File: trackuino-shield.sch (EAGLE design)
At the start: 19 parts, among them IC2 AP1117, M1 HX1, Q1 IRLD110, U1 LM60 int, X1 BU-SMA-V, X2 Vin, X3 LM60 ext, X4 Buzzer

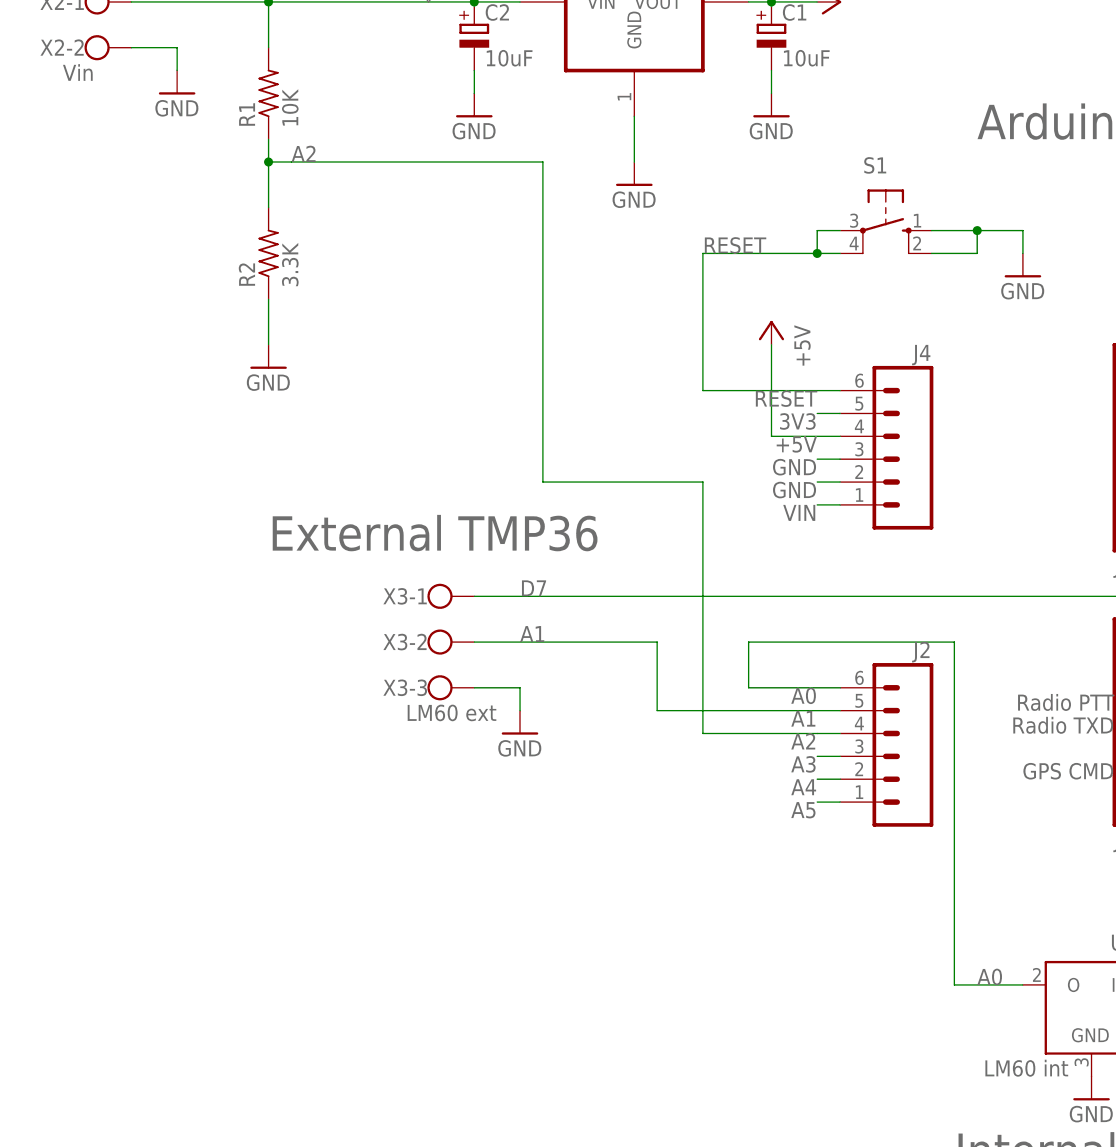
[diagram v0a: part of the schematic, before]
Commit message: Added logo
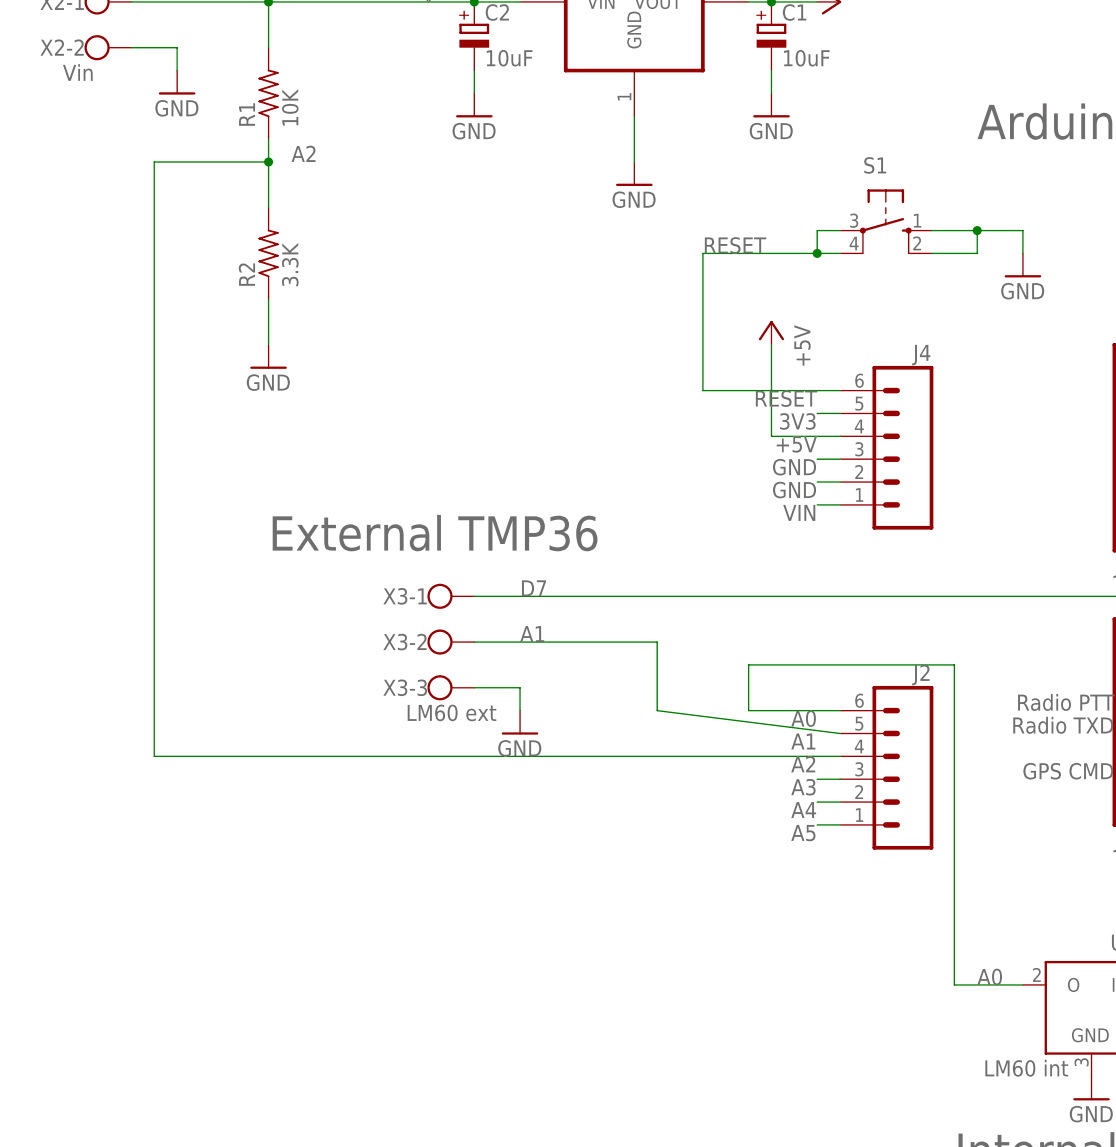
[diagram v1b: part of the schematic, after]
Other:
- moved on the sheet: J2
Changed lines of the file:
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@@
 <instance part="S1" gate="1" x="99.06" y="137.16" rot="R270"/>
 <instance part="J4" gate="G$1" x="99.06" y="111.76" rot="MR0"/>
-<instance part="J2" gate="G$1" x="99.06" y="78.74" rot="MR0"/>
+<instance part="J2" gate="G$1" x="99.06" y="76.2" rot="MR0"/>
 <instance part="J3" gate="G$1" x="129.54" y="114.3" rot="MR180"/>
 <instance part="J1" gate="G$1" x="129.54" y="83.82" rot="MR180"/>
@@
 <pinref part="U1" gate="G$1" pin="O"/>
 <wire x1="114.3" y1="53.34" x2="106.68" y2="53.34" width="0.1524" layer="91"/>
-<wire x1="93.98" y1="86.36" x2="83.82" y2="86.36" width="0.1524" layer="91"/>
-<label x="91.44" y="86.36" size="1.778" layer="95" rot="R180"/>
+<wire x1="93.98" y1="83.82" x2="83.82" y2="83.82" width="0.1524" layer="91"/>
+<label x="91.44" y="83.82" size="1.778" layer="95" rot="R180"/>
 <pinref part="J2" gate="G$1" pin="6"/>
-<wire x1="106.68" y1="53.34" x2="106.68" y2="91.44" width="0.1524" layer="91"/>
-<wire x1="106.68" y1="91.44" x2="83.82" y2="91.44" width="0.1524" layer="91"/>
-<wire x1="83.82" y1="91.44" x2="83.82" y2="86.36" width="0.1524" layer="91"/>
+<wire x1="106.68" y1="53.34" x2="106.68" y2="88.9" width="0.1524" layer="91"/>
+<wire x1="106.68" y1="88.9" x2="83.82" y2="88.9" width="0.1524" layer="91"/>
+<wire x1="83.82" y1="88.9" x2="83.82" y2="83.82" width="0.1524" layer="91"/>
 </segment>
 </net>
@@
 <wire x1="53.34" y1="91.44" x2="73.66" y2="91.44" width="0.1524" layer="91"/>
 <wire x1="73.66" y1="91.44" x2="73.66" y2="83.82" width="0.1524" layer="91"/>
-<label x="91.44" y="83.82" size="1.778" layer="95" rot="R180"/>
+<label x="91.44" y="81.28" size="1.778" layer="95" rot="R180"/>
 <pinref part="J2" gate="G$1" pin="5"/>
-<wire x1="73.66" y1="83.82" x2="93.98" y2="83.82" width="0.1524" layer="91"/>
+<wire x1="73.66" y1="83.82" x2="93.98" y2="81.28" width="0.1524" layer="91"/>
 </segment>
 </net>
@@
 <wire x1="30.48" y1="147.32" x2="30.48" y2="144.78" width="0.1524" layer="91"/>
 <wire x1="30.48" y1="144.78" x2="30.48" y2="139.7" width="0.1524" layer="91"/>
-<wire x1="30.48" y1="144.78" x2="33.02" y2="144.78" width="0.1524" layer="91"/>
 <junction x="30.48" y="144.78"/>
 <label x="33.02" y="144.78" size="1.778" layer="95"/>
 <pinref part="R1" gate="G$1" pin="1"/>
 <pinref part="R2" gate="G$1" pin="2"/>
-<wire x1="33.02" y1="144.78" x2="60.96" y2="144.78" width="0.2032" layer="91"/>
-<wire x1="60.96" y1="144.78" x2="60.96" y2="109.22" width="0.2032" layer="91"/>
-<wire x1="60.96" y1="109.22" x2="78.74" y2="109.22" width="0.2032" layer="91"/>
-<wire x1="78.74" y1="109.22" x2="78.74" y2="81.28" width="0.2032" layer="91"/>
-<wire x1="78.74" y1="81.28" x2="91.44" y2="81.28" width="0.2032" layer="91"/>
-<wire x1="93.98" y1="81.28" x2="91.44" y2="81.28" width="0.1524" layer="91"/>
-<label x="91.44" y="81.28" size="1.778" layer="95" rot="R180"/>
+<wire x1="30.48" y1="144.78" x2="17.78" y2="144.78" width="0.1524" layer="91"/>
+<wire x1="17.78" y1="144.78" x2="17.78" y2="78.74" width="0.1524" layer="91"/>
+<wire x1="17.78" y1="78.74" x2="93.98" y2="78.74" width="0.1524" layer="91"/>
+<label x="91.44" y="78.74" size="1.778" layer="95" rot="R180"/>
 <pinref part="J2" gate="G$1" pin="4"/>
 </segment>
 </net>
 <net name="A3" class="0">
-<segment>
-<wire x1="93.98" y1="78.74" x2="91.44" y2="78.74" width="0.1524" layer="91"/>
-<label x="91.44" y="78.74" size="1.778" layer="95" rot="R180"/>
-<pinref part="J2" gate="G$1" pin="3"/>
-</segment>
-</net>
-<net name="A4" class="0">
 <segment>
 <wire x1="93.98" y1="76.2" x2="91.44" y2="76.2" width="0.1524" layer="91"/>
 <label x="91.44" y="76.2" size="1.778" layer="95" rot="R180"/>
-<pinref part="J2" gate="G$1" pin="2"/>
-</segment>
-</net>
-<net name="A5" class="0">
+<pinref part="J2" gate="G$1" pin="3"/>
+</segment>
+</net>
+<net name="A4" class="0">
 <segment>
 <wire x1="93.98" y1="73.66" x2="91.44" y2="73.66" width="0.1524" layer="91"/>
 <label x="91.44" y="73.66" size="1.778" layer="95" rot="R180"/>
+<pinref part="J2" gate="G$1" pin="2"/>
+</segment>
+</net>
+<net name="A5" class="0">
+<segment>
+<wire x1="93.98" y1="71.12" x2="91.44" y2="71.12" width="0.1524" layer="91"/>
+<label x="91.44" y="71.12" size="1.778" layer="95" rot="R180"/>
 <pinref part="J2" gate="G$1" pin="1"/>
 </segment>
